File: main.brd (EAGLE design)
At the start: 23.6 x 22.9 mm, 23 parts, among them Q1 BSS84, U1 433MHz, U2 ATMEGA328P-MU-QFN32

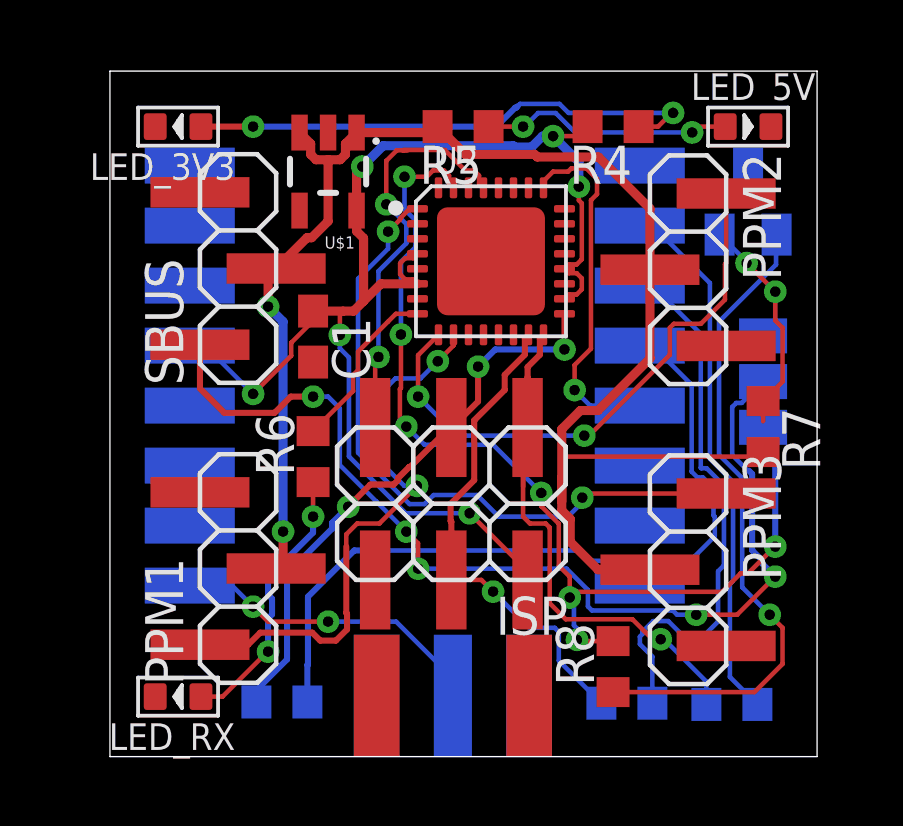
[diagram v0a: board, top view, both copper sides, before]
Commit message: Started redesign
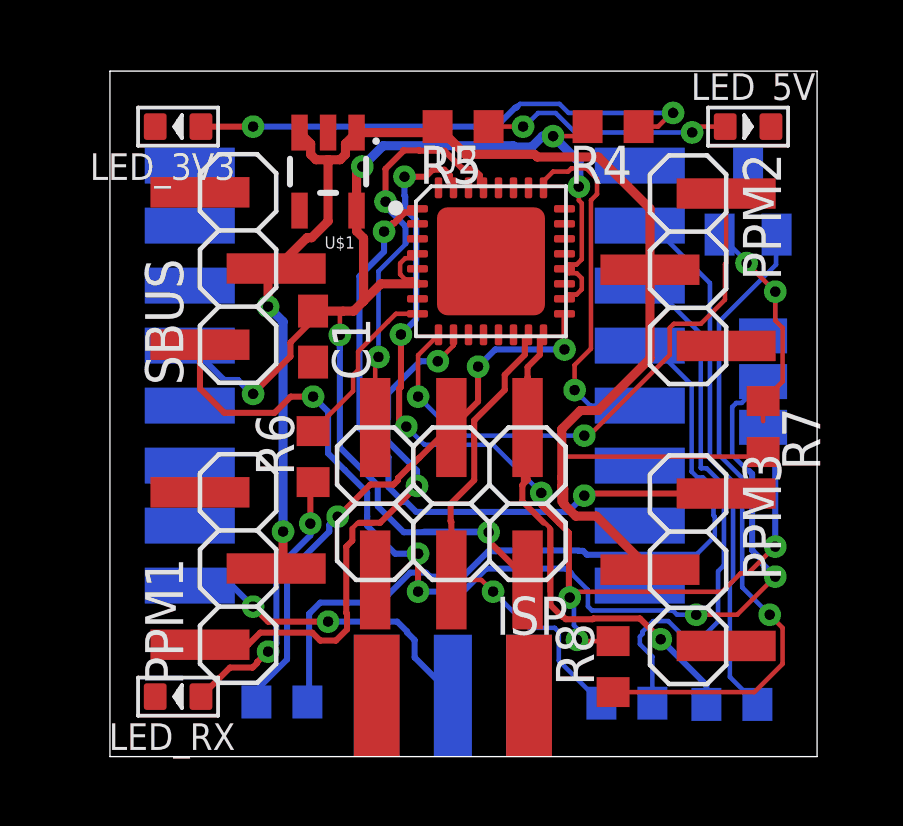
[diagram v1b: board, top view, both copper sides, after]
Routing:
- net +3V3: track 44.6 -> 47.6 mm
- net !SBUS: track 34.6 -> 37.6 mm
- net N$2: track 25.9 -> 28.4 mm
- net N$6: track 34.3 -> 36.3 mm
- net MISO: track 22.6 -> 24.3 mm
- net SCK: track 22.5 -> 21.1 mm
- net +5V: track 52.8 -> 51.8 mm
- net PPM1: track 19.2 -> 18.6 mm
